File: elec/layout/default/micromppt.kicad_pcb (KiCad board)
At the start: 2 copper layers, 29 x 28.5 mm, 19 parts, among them J1 ?, J2 ?, U1 ?, U2 ?, U3 ?, U4 ?, U5 ?

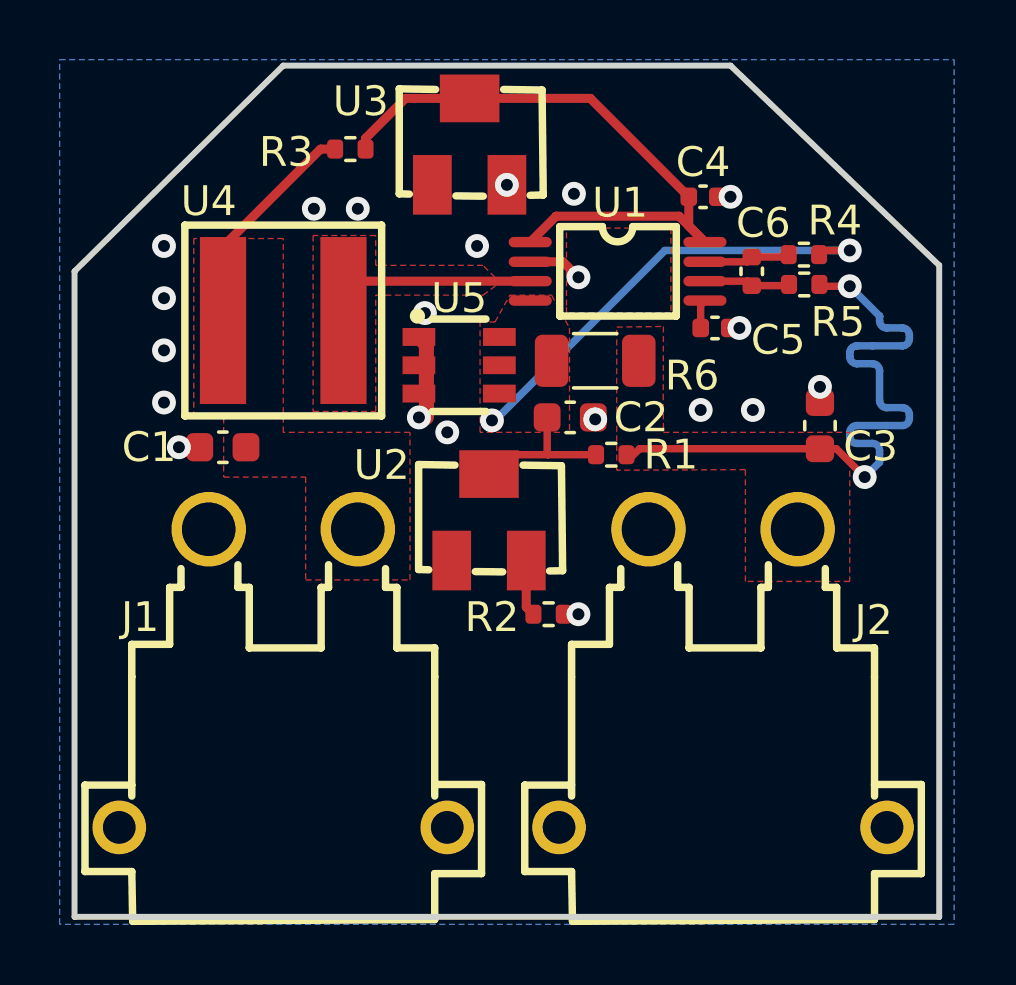
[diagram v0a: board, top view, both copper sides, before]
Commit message: MICROMPPT V2
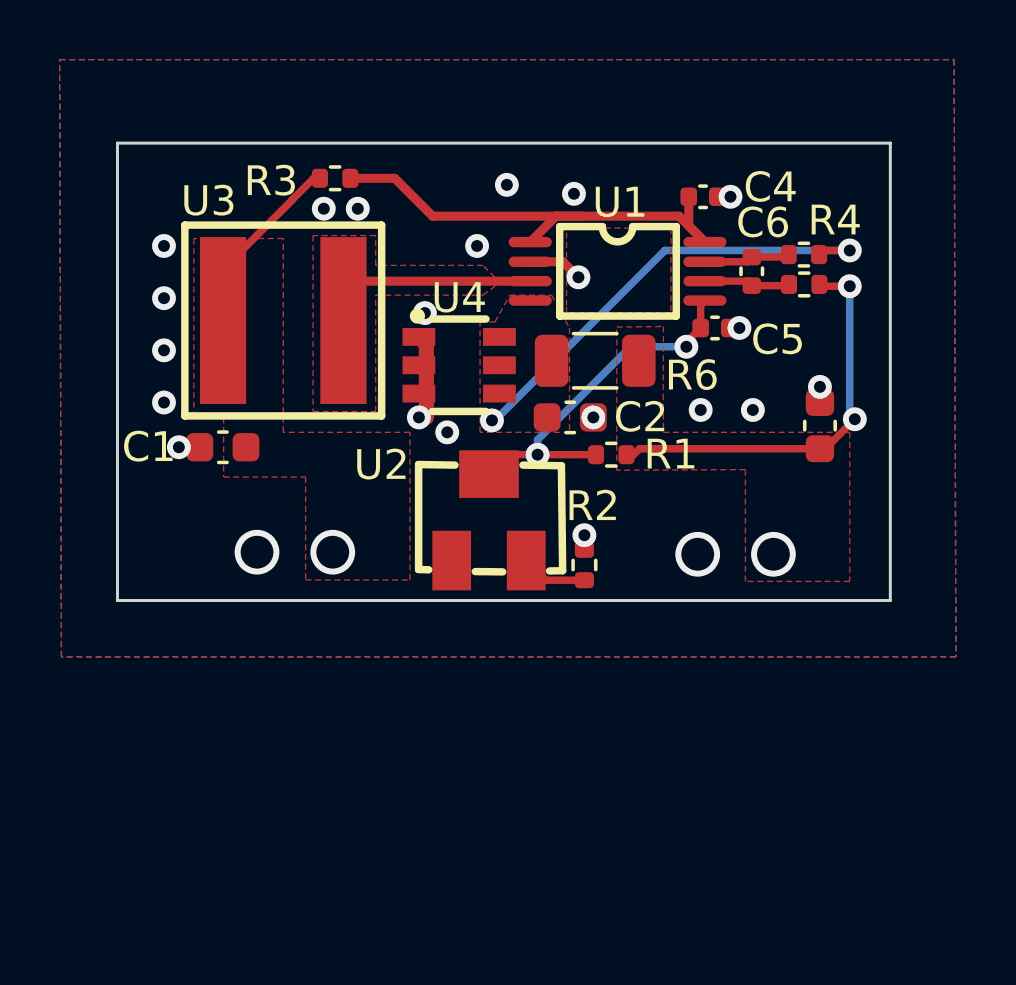
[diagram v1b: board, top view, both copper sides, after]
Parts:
- removed J1, J2: ?, lib:CONN-TH_XT30PW-M
- removed the U3 at (78.2, 41.8)
- moved R2 2.04 mm to (82.1, 56.0), turned to 90 degrees
- moved R3 1.10 mm to (73.7, 43.0)
- renumbered U4 to U3, U5 to U4
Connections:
- net VR2-p1 renamed p1
- R1 pad 2: vout -> vctrl
- U2 pad 2: vout -> vctrl
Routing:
- net vctrl: track 0.98 -> 13.0 mm, vias 0 -> 2
- net vcc-2: track 23.4 -> 13.7 mm, vias 2 -> 3
- net vout: track 21.1 -> 15.4 mm
- net xshut: track 21.4 -> 16.7 mm
- net vcc-1: track 7.59 -> 8.72 mm, vias 0 -> 1
- net gnd: vias 21 -> 23
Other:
- board size 29 x 28.5 mm -> 25.9 x 15.3 mm
